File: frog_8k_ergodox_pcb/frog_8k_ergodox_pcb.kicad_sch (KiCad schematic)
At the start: 214 parts, among them J1 USB_C_Receptacle_USB2.0_14P, J10 Conn_01x01_Pin, J2 Conn_01x04_Pin, J3 Conn_01x01_Pin, J4 Conn_01x01_Pin, J5 Conn_01x01_Pin, J6 Conn_01x01_Pin, J7 Conn_01x01_Pin, J8 Conn_01x01_Pin, J9 Conn_01x01_Pin, SW1 SW_DPST_x2, SW2 SW_DPST_x2, U1 PMW3360DM-T2QU, U2 STM32F072CBTx, U3 TLV74318PDBVR, U4 XC6206PxxxMR, U5 SRV05-4

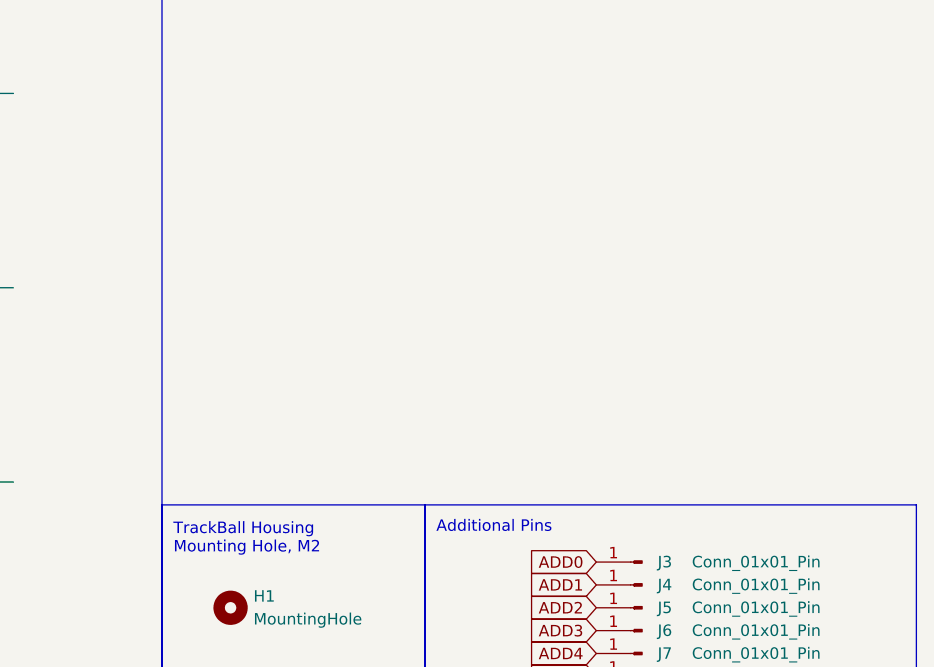
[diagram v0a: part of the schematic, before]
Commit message: Almost Done with pcb
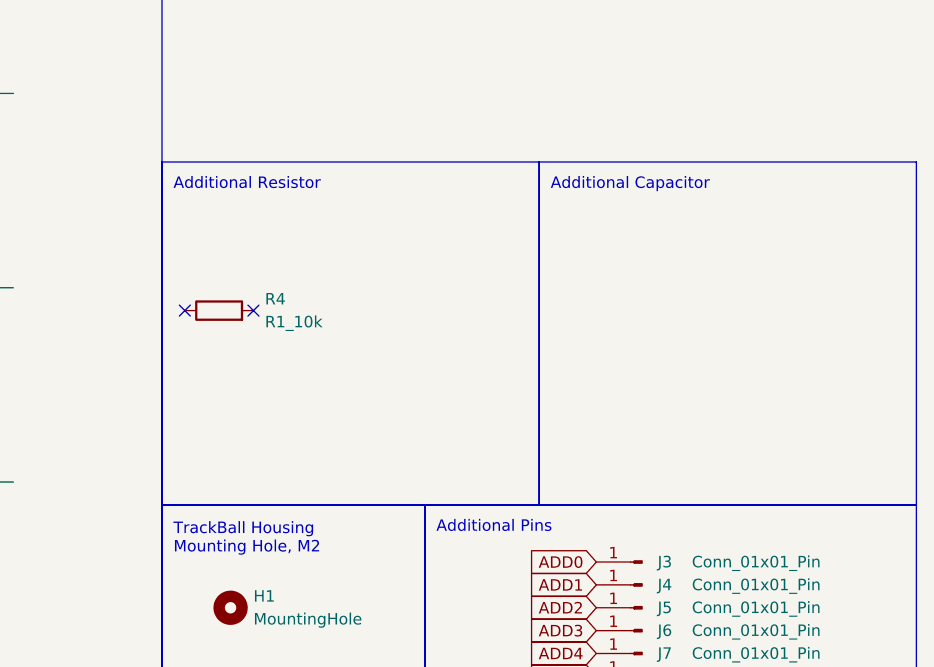
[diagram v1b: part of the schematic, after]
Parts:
- added R4: R1_10k, Resistor_SMD:R_0805_2012Metric_Pad1.20x1.40mm_HandSolder, symbol Device:R
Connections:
- no-connect marks 4 -> 6
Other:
- note added: "Additional Capacitor"
- note added: "Additional Resistor"
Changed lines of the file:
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@@
 	)
 	(no_connect
+		(at 326.39 77.47)
+	)
+	(no_connect
+		(at 334.01 77.47)
+	)
+	(no_connect
 		(at 270.51 261.62)
 	)
@@
 	)
 	(rectangle
+		(start 323.85 60.96)
+		(end 365.76 99.06)
+		(stroke
+			(width 0)
+			(type default)
+		)
+		(fill
+			(type none)
+		)
+	)
+	(rectangle
 		(start 212.09 237.49)
 		(end 299.72 284.48)
@@
 		)
 	)
+	(rectangle
+		(start 365.76 60.96)
+		(end 407.67 99.06)
+		(stroke
+			(width 0)
+			(type default)
+		)
+		(fill
+			(type none)
+		)
+	)
 	(text "TrackBall Housing\nMounting Hole, M2"
 		(exclude_from_sim no)
@@
 		)
 	)
+	(text "Additional Resistor"
+		(exclude_from_sim no)
+		(at 325.12 63.5 0)
+		(effects
+			(font
+				(size 1.27 1.27)
+			)
+			(justify left)
+		)
+	)
 	(text "MCU STM32F072CBT6"
 		(exclude_from_sim no)
@@
 		)
 	)
+	(text "Additional Capacitor"
+		(exclude_from_sim no)
+		(at 367.03 63.5 0)
+		(effects
+			(font
+				(size 1.27 1.27)
+			)
+			(justify left)
+		)
+	)
 	(text "Boot Switch\n"
 		(exclude_from_sim no)
@@
 					(unit 1)
 				)
+			)
+		)
+	)
+	(symbol
+		(lib_id "Device:R")
+		(at 330.2 77.47 90)
+		(unit 1)
+		(exclude_from_sim no)
+		(in_bom yes)
+		(on_board yes)
+		(dnp no)
+		(property "Reference" "R4"
+			(at 335.28 76.2 90)
+			(effects
+				(font
+					(size 1.27 1.27)
+				)
+				(justify right)
+			)
+		)
+		(property "Value" "R1_10k"
+			(at 335.28 78.74 90)
+			(effects
+				(font
+					(size 1.27 1.27)
+				)
+				(justify right)
+			)
+		)
+		(property "Footprint" "Resistor_SMD:R_0805_2012Metric_Pad1.20x1.40mm_HandSolder"
+			(at 330.2 79.248 90)
+			(effects
+				(font
+					(size 1.27 1.27)
+				)
+				(hide yes)
+			)
+		)
+		(property "Datasheet" "~"
+			(at 330.2 77.47 0)
+			(effects
+				(font
+					(size 1.27 1.27)
+				)
+				(hide yes)
+			)
+		)
+		(property "Description" "Resistor"
+			(at 330.2 77.47 0)
+			(effects
+				(font
+					(size 1.27 1.27)
+				)
+				(hide yes)
+			)
+		)
+		(pin "1"
+		)
+		(pin "2"
+		)
+		(instances
+			(project "frog_8k_ergodox_pcb"
+				(path "/34ddd234-11af-4a66-9186-ea72bce9a0a9"
+					(reference "R4")
+					(unit 1)
+				)
